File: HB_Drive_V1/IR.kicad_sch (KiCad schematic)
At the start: 53 parts, among them J15 Conn_02x04_Counter_Clockwise, J5 Conn_02x03_Counter_Clockwise, J6 Conn_01x02, U22 TL082, U23 TL082, U4 TL082, U5 TL082, U6 TL082, U8 TL082

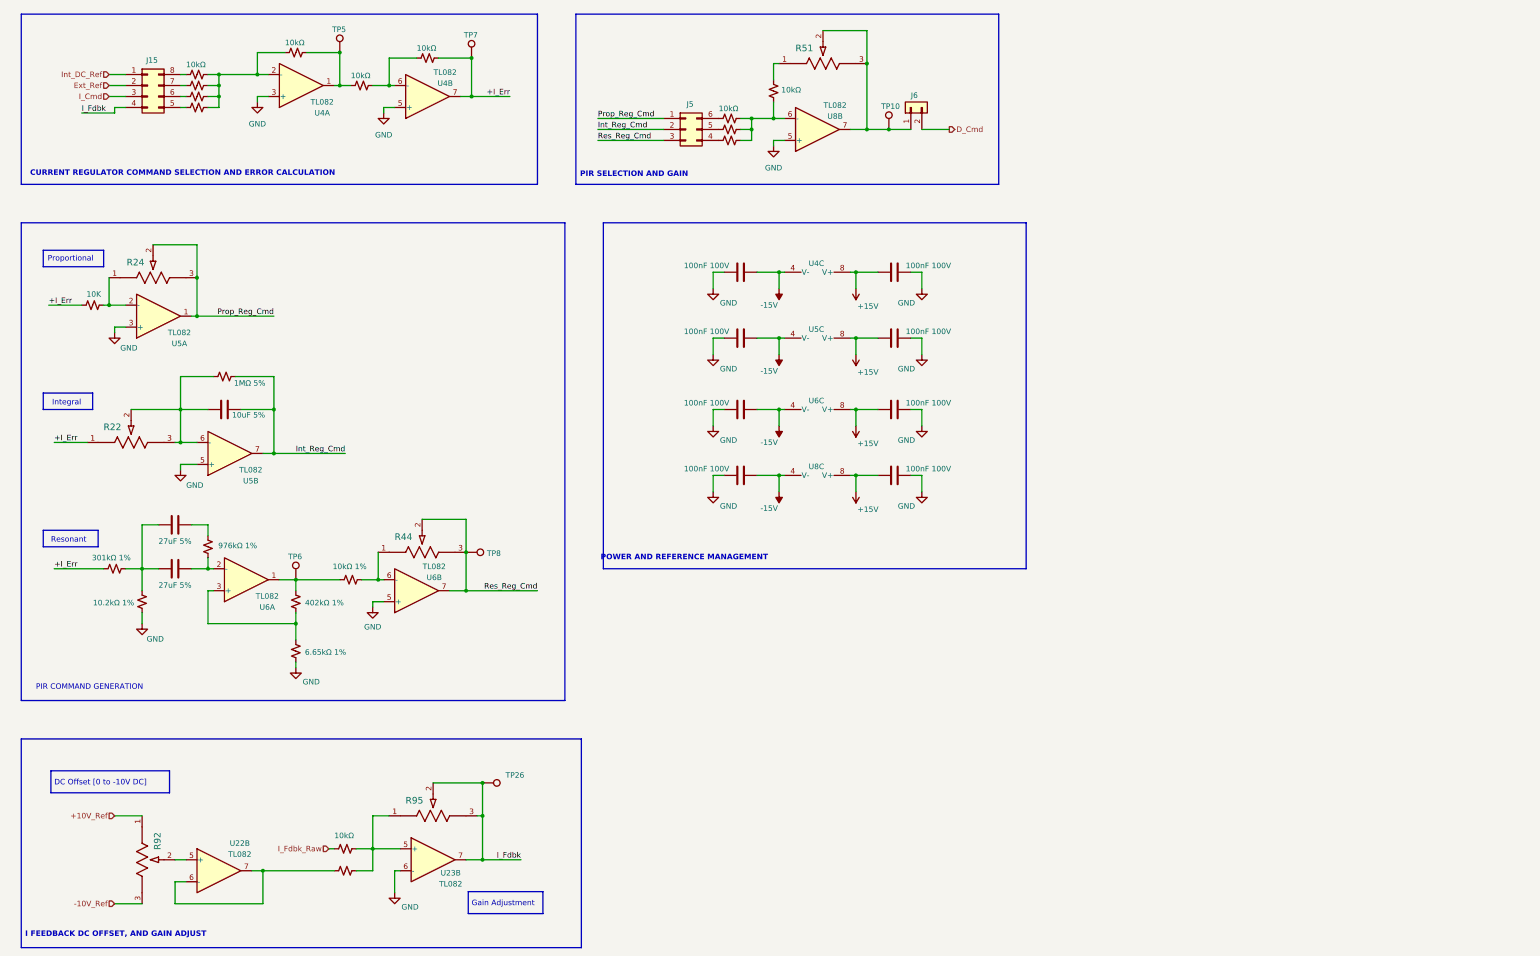
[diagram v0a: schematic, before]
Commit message: updates board to highest working copy
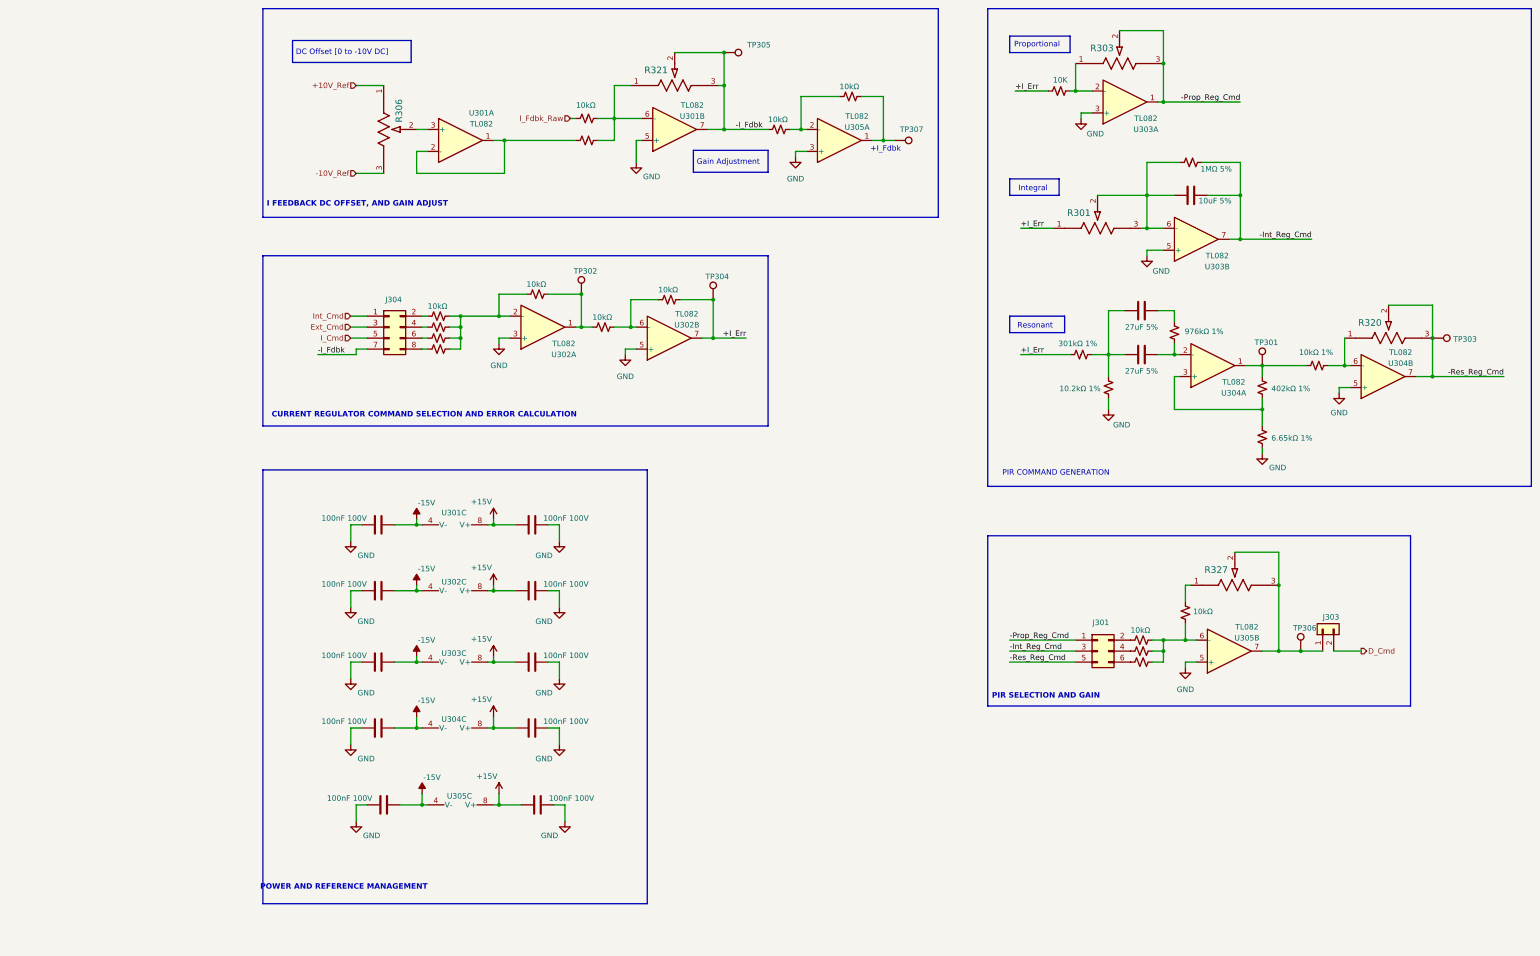
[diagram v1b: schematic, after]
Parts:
- removed C11, C12, C13, C14, C15, C16, C17, C18: 100nF 100V, Capacitor_SMD:C_0603_1608Metric, symbol Device:C
- removed J15: Conn_02x04_Counter_Clockwise, Connector_PinSocket_1.27mm:PinSocket_2x04_P1.27mm_Vertical, symbol Connector_Generic:Conn_02x04_Counter_Clockwise
- removed J5: Conn_02x03_Counter_Clockwise, Connector_PinSocket_1.27mm:PinSocket_2x03_P1.27mm_Vertical, symbol Connector_Generic:Conn_02x03_Counter_Clockwise
- removed U23: TL082, symbol Amplifier_Operational:TL082
- removed unit 3 of U4
- removed unit 3 of U5
- removed unit 3 of U6
- removed unit 3 of U8
- added C304, C305, C306, C307, C308, C309, C310, C311, C312, C313: 100nF 100V, Capacitor_SMD:C_0603_1608Metric, symbol Device:C
- added J301: Conn_02x03_Odd_Even, Connector_PinHeader_2.54mm:PinHeader_2x03_P2.54mm_Vertical, symbol Connector_Generic:Conn_02x03_Odd_Even
- added J304: Conn_02x04_Odd_Even, Connector_PinHeader_2.54mm:PinHeader_2x04_P2.54mm_Vertical, symbol Connector_Generic:Conn_02x04_Odd_Even
- added R328, R329: 10kΩ, Resistor_SMD:R_0603_1608Metric_Pad0.98x0.95mm_HandSolder, symbol Device:R_Small_US
- added TP307: TestPoint, TestPoint:TestPoint_Loop_D2.60mm_Drill1.6mm_Beaded, symbol Connector:TestPoint
- added unit 2 of U301
- added unit 3 of U301
- added unit 3 of U302
- added unit 3 of U303
- added unit 3 of U304
- added unit 1 of U305
- added unit 3 of U305
- U301: renamed from U22; footprint Package_SO:SOIC-8_5.3x5.3mm_P1.27mm -> Package_SO:SOIC-8_3.9x4.9mm_P1.27mm
- U302: renamed from U4; footprint (none) -> Package_SO:SOIC-8_3.9x4.9mm_P1.27mm
- U303: renamed from U5; footprint Package_SO:SOIC-8_5.3x5.3mm_P1.27mm -> Package_SO:SOIC-8_3.9x4.9mm_P1.27mm
- U304: renamed from U6; footprint (none) -> Package_SO:SOIC-8_3.9x4.9mm_P1.27mm
- U305: renamed from U8; footprint (none) -> Package_SO:SOIC-8_3.9x4.9mm_P1.27mm
- renumbered C8 to C301, C9 to C302, C10 to C303, J6 to J303, R22 to R301, R23 to R302, R24 to R303, R25 to R304, R27 to R305, R92 to R306, R28 to R307, R29 to R308, R30 to R309, R31 to R310, R34 to R311, R35 to R312, R26 to R313, R38 to R314, R39 to R315, R93 to R316, R94 to R317, R42 to R318, R33 to R319, R44 to R320, R95 to R321, R37 to R322, R47 to R323, R48 to R324, R49 to R325, R50 to R326, R51 to R327, TP6 to TP301, TP5 to TP302, TP8 to TP303, TP7 to TP304, TP26 to TP305, TP10 to TP306
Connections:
- net +15V: now also C306.2, C307.2, C310.2, C311.2, C313.2, U301.8 (V+), U302.8 (V+), U303.8 (V+), U304.8 (V+), U305.8 (V+)
- net -15V: now also C304.1, C305.1, C308.1, C309.1, C312.1, U301.4 (V-), U302.4 (V-), U303.4 (V-), U304.4 (V-), U305.4 (V-)
- net GND: now also C304.2, C305.2, C306.1, C307.1, C308.2, C309.2, C310.1, C311.1, C312.2, C313.1, U301.5 (+), U305.3 (+)
- net I_Cmd: now also J304.5 (Pin_5)
- net at R310.1: now also J304.8 (Pin_8)
- net at R316.1, R317.1, R321.1: now also U301.6 (-)
- net at R325.1: now also J301.6 (Pin_6)
- net at R324.1: now also J301.4 (Pin_4)
- net at R323.2: now also J301.2 (Pin_2)
- net at R307.2: now also J304.2 (Pin_2)
- net at R308.1: now also J304.4 (Pin_4)
- net at R309.1: now also J304.6 (Pin_6)
- net at R306.2: now also U301.3 (+); no longer U301.5 (+)
- net I_Fdbk renamed -I_Fdbk
- net -I_Fdbk: now also J304.7 (Pin_7), R328.2, U301.7
- net Int_Reg_Cmd renamed -Int_Reg_Cmd
- net -Int_Reg_Cmd: now also J301.3 (Pin_3)
- net Prop_Reg_Cmd renamed -Prop_Reg_Cmd
- net -Prop_Reg_Cmd: now also J301.1 (Pin_1)
- net Res_Reg_Cmd renamed -Res_Reg_Cmd
- net -Res_Reg_Cmd: now also J301.5 (Pin_5)
- new net: R329.1, TP307.1, U305.1
- new net: R328.1, R329.2, U305.2 (-)
- new net: R317.2, U301.1, U301.2 (-)
- new net Ext_Cmd: J304.3 (Pin_3)
- new net Int_Cmd: J304.1 (Pin_1)
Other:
- note added: "+I_Fdbk"
- moved on the sheet: J303, R301, R303, R306, R320, R321, R327, TP301, TP302, TP303, TP304, TP305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
